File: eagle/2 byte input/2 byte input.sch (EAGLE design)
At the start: 26 parts, among them IC1 74LS165N, IC2 74LS165N, X1 MKDSN1,5/5-5,08, X2 MKDSN1,5/5-5,08, X3 MKDSN1,5/8-5,08, X5 MKDSN1,5/8-5,08

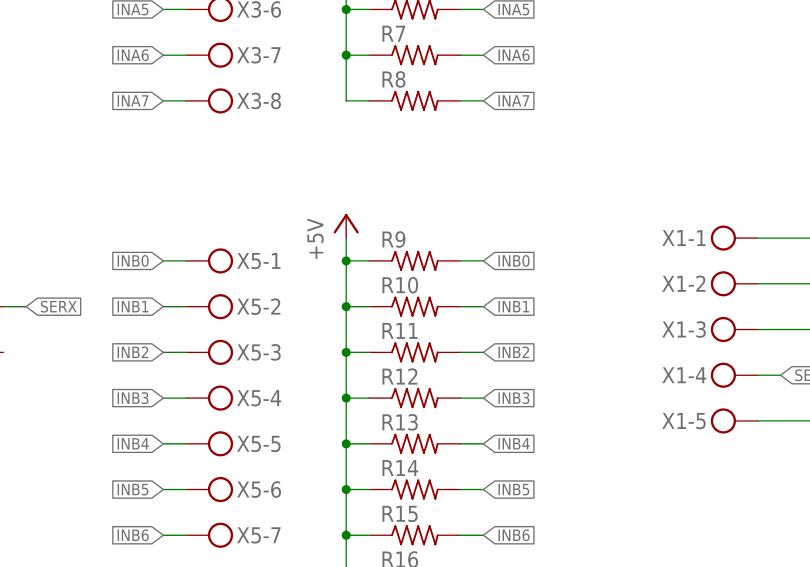
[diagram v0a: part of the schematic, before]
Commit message: check in changes
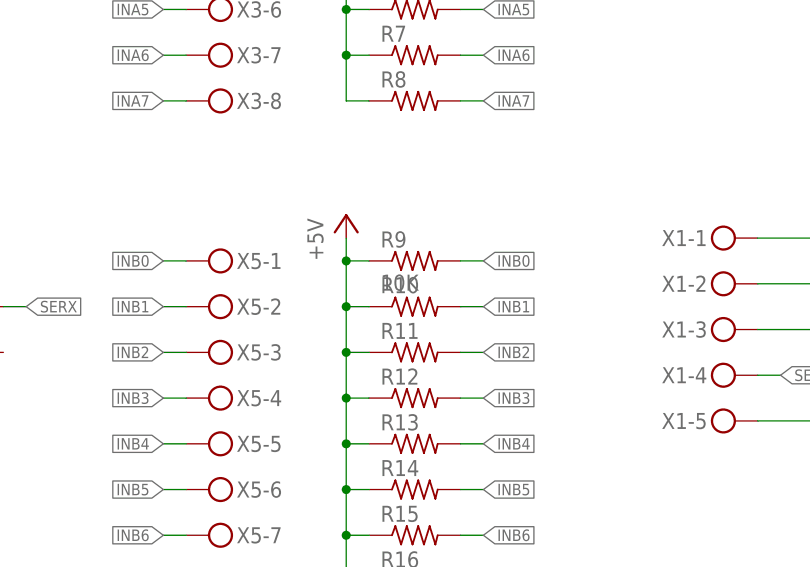
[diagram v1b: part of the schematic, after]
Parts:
- R9: value (none) -> 10K
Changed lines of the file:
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@@
 <part name="R7" library="resistor" library_urn="urn:adsk.eagle:library:348" deviceset="R-US_" device="0207/2V" package3d_urn="urn:adsk.eagle:package:23490/1"/>
 <part name="R8" library="resistor" library_urn="urn:adsk.eagle:library:348" deviceset="R-US_" device="0207/2V" package3d_urn="urn:adsk.eagle:package:23490/1"/>
-<part name="R9" library="resistor" library_urn="urn:adsk.eagle:library:348" deviceset="R-US_" device="0207/2V" package3d_urn="urn:adsk.eagle:package:23490/1"/>
+<part name="R9" library="resistor" library_urn="urn:adsk.eagle:library:348" deviceset="R-US_" device="0207/2V" package3d_urn="urn:adsk.eagle:package:23490/1" value="10K"/>
 <part name="R10" library="resistor" library_urn="urn:adsk.eagle:library:348" deviceset="R-US_" device="0207/2V" package3d_urn="urn:adsk.eagle:package:23490/1"/>
 <part name="R11" library="resistor" library_urn="urn:adsk.eagle:library:348" deviceset="R-US_" device="0207/2V" package3d_urn="urn:adsk.eagle:package:23490/1"/>
